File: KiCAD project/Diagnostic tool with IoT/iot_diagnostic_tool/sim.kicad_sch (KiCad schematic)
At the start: 11 parts, among them J1 SIM7050-8-0-00-X_REVC

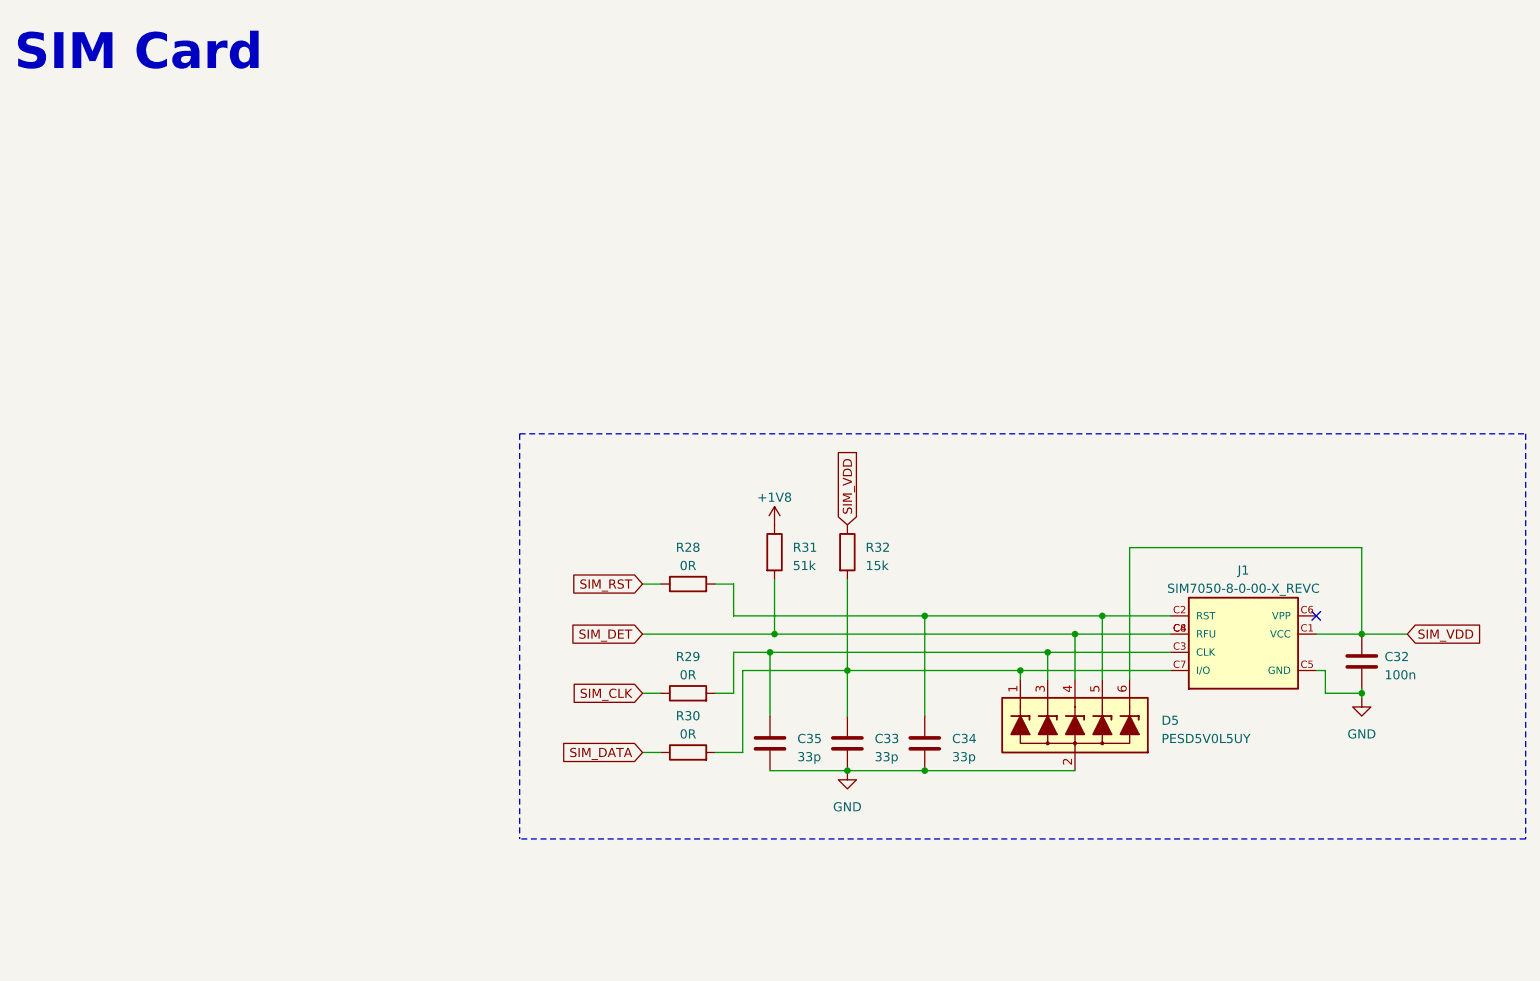
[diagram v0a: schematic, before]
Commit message: Update 06/03/23 - new board layout WIP 70%
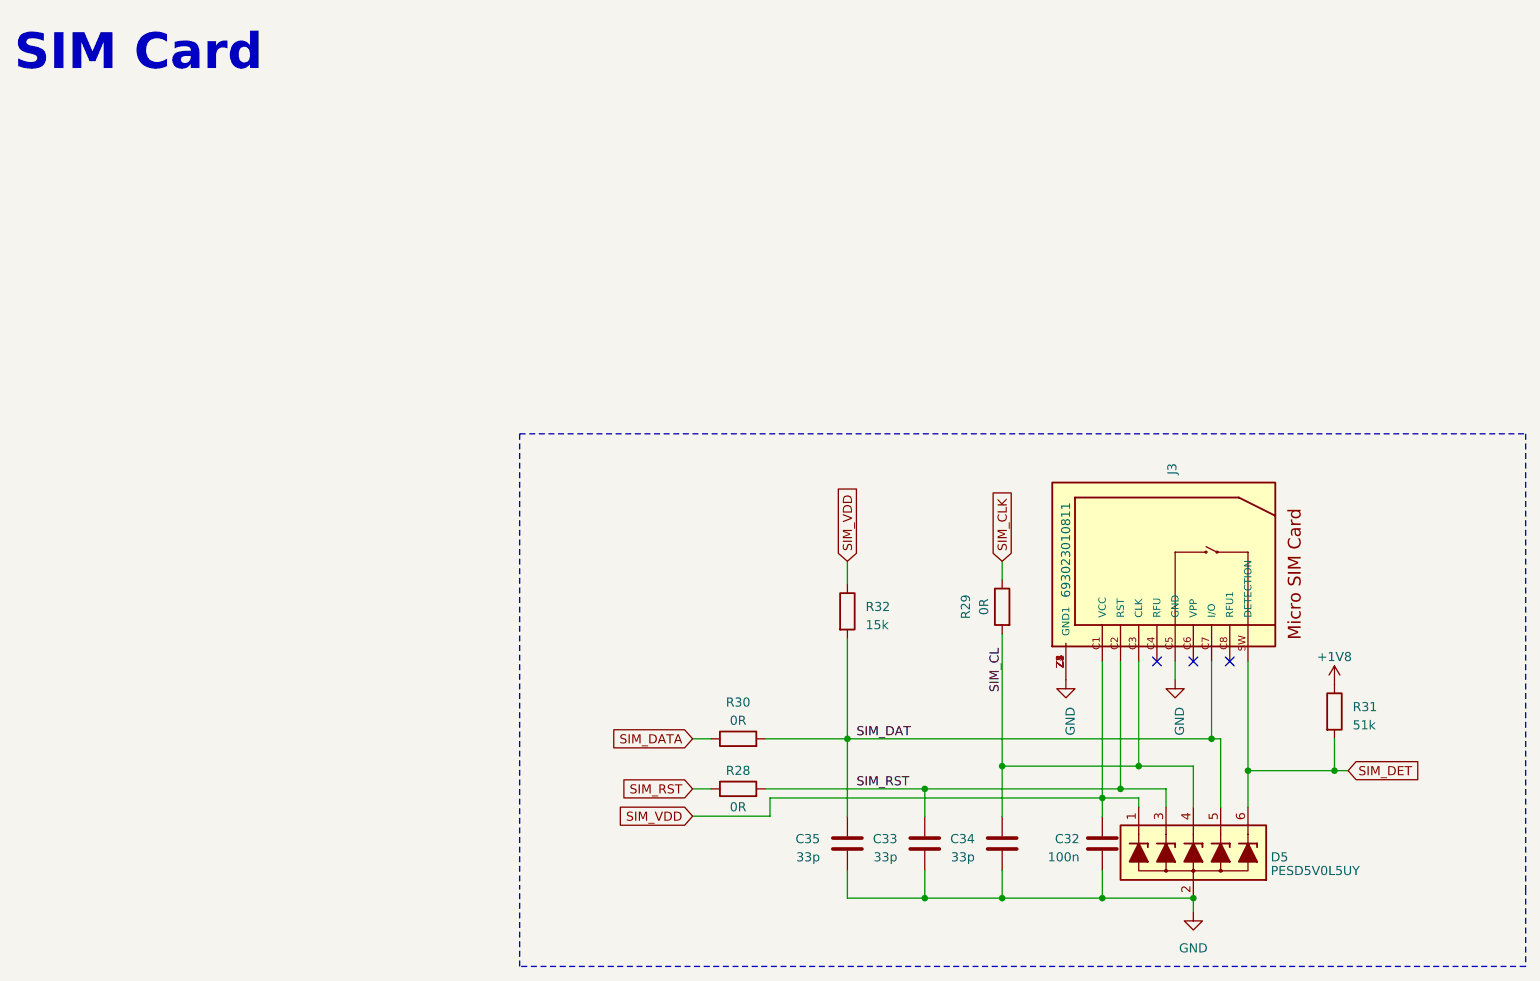
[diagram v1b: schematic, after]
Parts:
- removed J1: SIM7050-8-0-00-X_REVC, GCT_SIM7050-8-0-00-X_REVC, symbol SIM7050-8-0-00-X_REVC:SIM7050-8-0-00-X_REVC
- added J3: 693023010811, 693023010811, symbol 693023010811:693023010811
- C32, C33, C34, C35: footprint (none) -> Capacitor_SMD:C_0402_1005Metric
- D5: footprint Package_TO_SOT_SMD_AKL:SOT-363_SC-70-6 -> Package_TO_SOT_SMD:SOT-363_SC-70-6
- R28, R29, R30, R31, R32: footprint (none) -> Resistor_SMD:R_0402_1005Metric
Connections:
- net GND: now also J3.C5 (GND), J3.Z1 (GND1), J3.Z2 (GND1), J3.Z3 (GND1), J3.Z4 (GND1), J3.Z5 (GND1)
- net SIM_DET: now also D5.6 (L5), J3.SW (DETECTION); no longer D5.4 (L3)
- net SIM_RST: now also C33.1, D5.3 (L2), R28.2, J3.C2 (RST)
- net SIM_VDD: now also D5.1 (L1), J3.C1 (VCC); no longer D5.6 (L5)
- net SIM_DAT: now reaches R30.2, R32.2
- net SIM_DAT: now also C35.1, D5.5 (L4), J3.C7 (I/O); no longer C33.1, D5.1 (L1)
- new net SIM_CL: C34.1, D5.4 (L3), J3.C3 (CLK), R29.2
- no-connect marks 1 -> 3
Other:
- moved on the sheet: C32, C33, C34, C35, D5, R28, R29, R30, R31, R32
